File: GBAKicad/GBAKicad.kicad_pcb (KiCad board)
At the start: 2 copper layers, 63 parts, among them J1 USB_C_Receptacle_USB2.0_16P, J2 BATT_Conn, J3 Jumper, J4 OLED_Conn, Q2 PMOS, SW1 EN, SW10 BTN_R, SW11 BTN_X, SW12 BTN_A, SW13 BTN_B, SW14 BTN_Y, SW15 BTN_SELECT, SW16 BTN_SYS, SW2 SW_PWR, SW3 BOOT, SW4 BTN_L, SW5 BTN_UP, SW6 BTN_LEFT, SW7 BTN_DOWN, SW8 BTN_RIGHT, SW9 BTN_START, U1 ESP32-S3-WROOM-1, U2 MIC5219-3.3YM5, U3 TP4056-42-ESOP8, U4 DW01A, U5 AMS1117-3.3

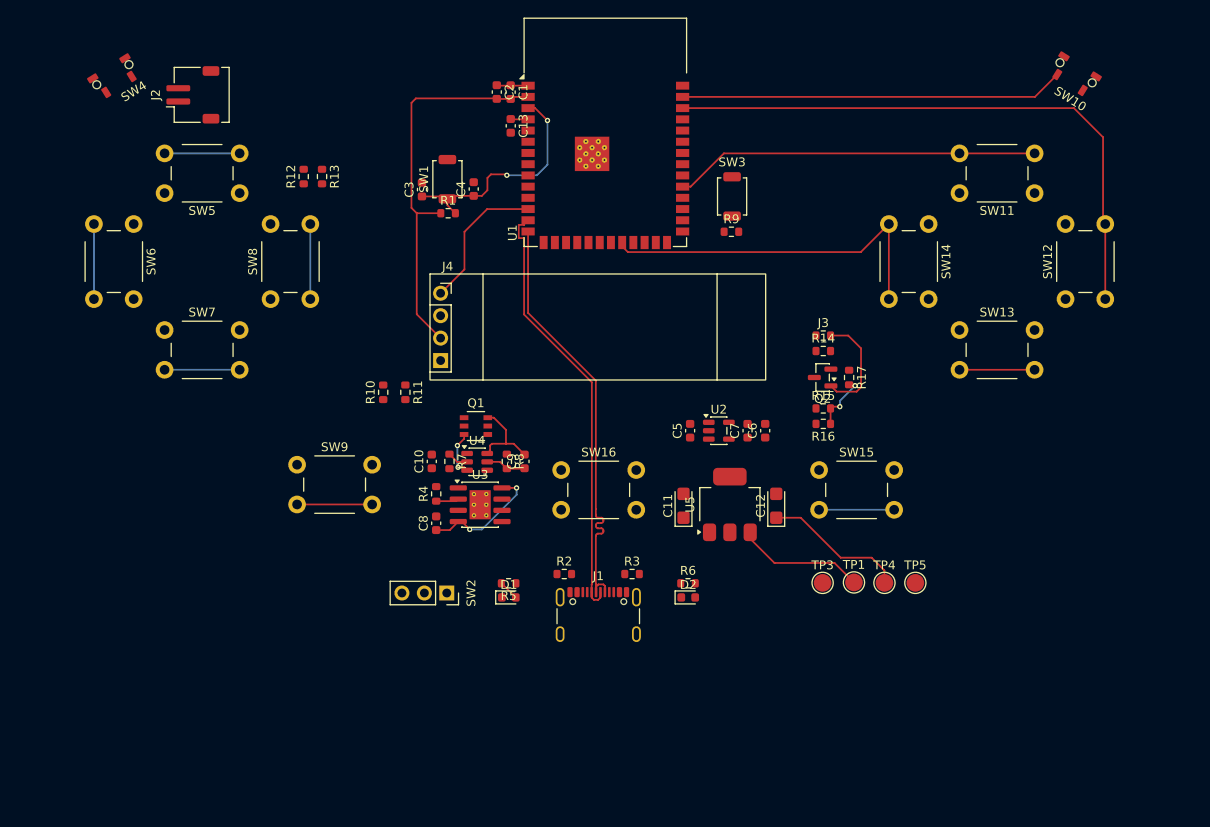
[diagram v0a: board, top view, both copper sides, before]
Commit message: pcb change
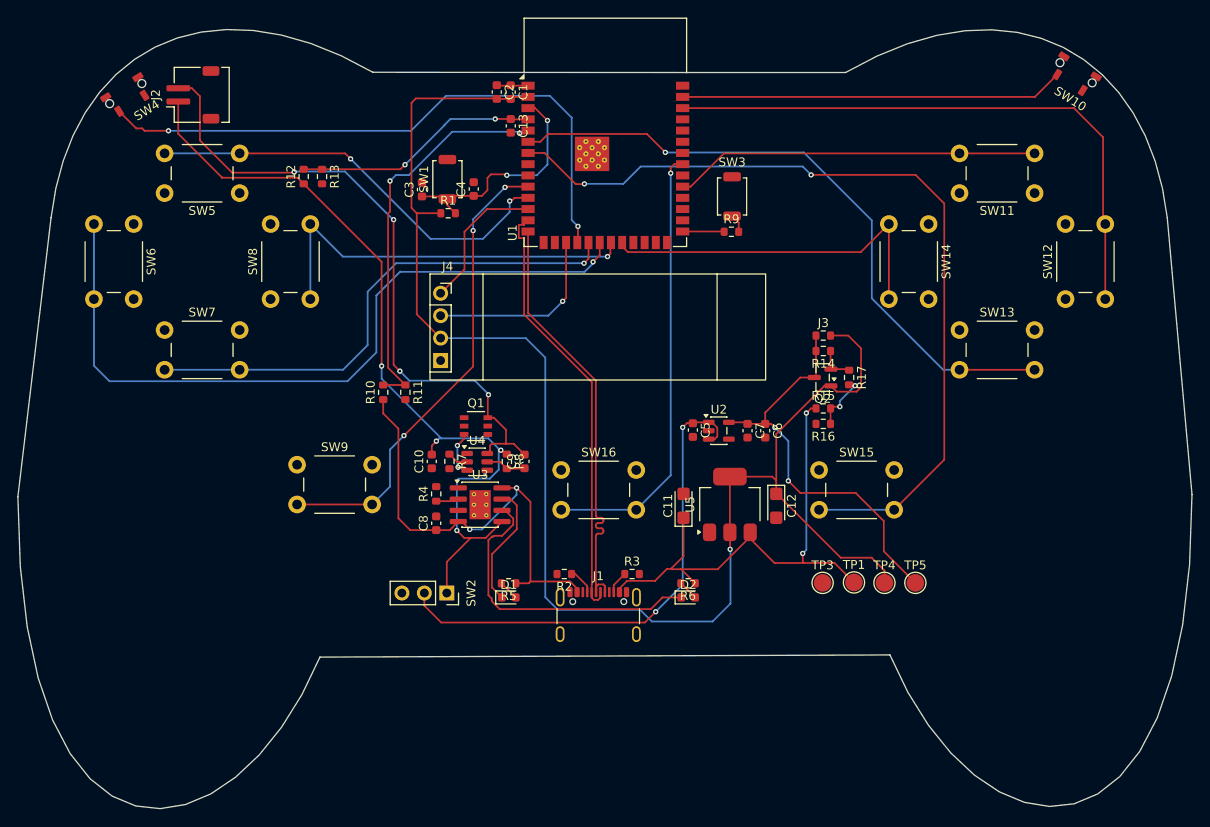
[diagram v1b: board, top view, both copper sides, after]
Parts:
- moved SW4 2.59 mm to (96.0, 57.4)
- moved C5 0.32 mm to (161.1, 97.0), turned to -90 degrees
- turned C12 to -90 degrees
- turned C6 to -90 degrees
- turned C7 to -90 degrees
- turned R14 to 180 degrees
- turned R2 to 180 degrees
- turned R6 to 180 degrees
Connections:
- U1 pad 33: BTN_Sys -> BTN_SYS
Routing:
- net +3V3: track 72.7 -> 171.7 mm, vias 0 -> 1
- net OUT+: track 0.00 -> 93.0 mm, vias 0 -> 4
- net BTN_SELECT: track 8.50 -> 96.7 mm, vias 0 -> 2
- net +5V: track 28.4 -> 111.8 mm, vias 2 -> 4
- net BTN_LEFT: track 8.50 -> 85.3 mm, vias 0 -> 1
- net BTN_L: track 0.00 -> 69.3 mm, vias 0 -> 2
- net BTN_B: track 8.50 -> 73.9 mm, vias 0 -> 1
- net -BATT: track 9.73 -> 74.6 mm, vias 0 -> 4
- net Net-(SW2-B): track 0.00 -> 57.5 mm, vias 0 -> 2
- net BTN_SYS: track 0.00 -> 50.4 mm, vias 0 -> 1
- net BTN_DOWN: track 8.50 -> 58.6 mm, vias 0 -> 1
- net Net-(J3-A): track 0.00 -> 46.6 mm, vias 0 -> 2
- net BTN_START: track 8.50 -> 53.3 mm, vias 0 -> 3
- net CHRG_CHECK: track 0.00 -> 44.6 mm, vias 0 -> 2
- net BTN_UP: track 8.50 -> 47.8 mm, vias 0 -> 2
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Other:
- board outline added: 132.9 x 88.2 mm
